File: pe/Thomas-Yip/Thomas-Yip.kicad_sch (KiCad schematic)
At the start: 17 parts, among them U1 TPS563201DDCR

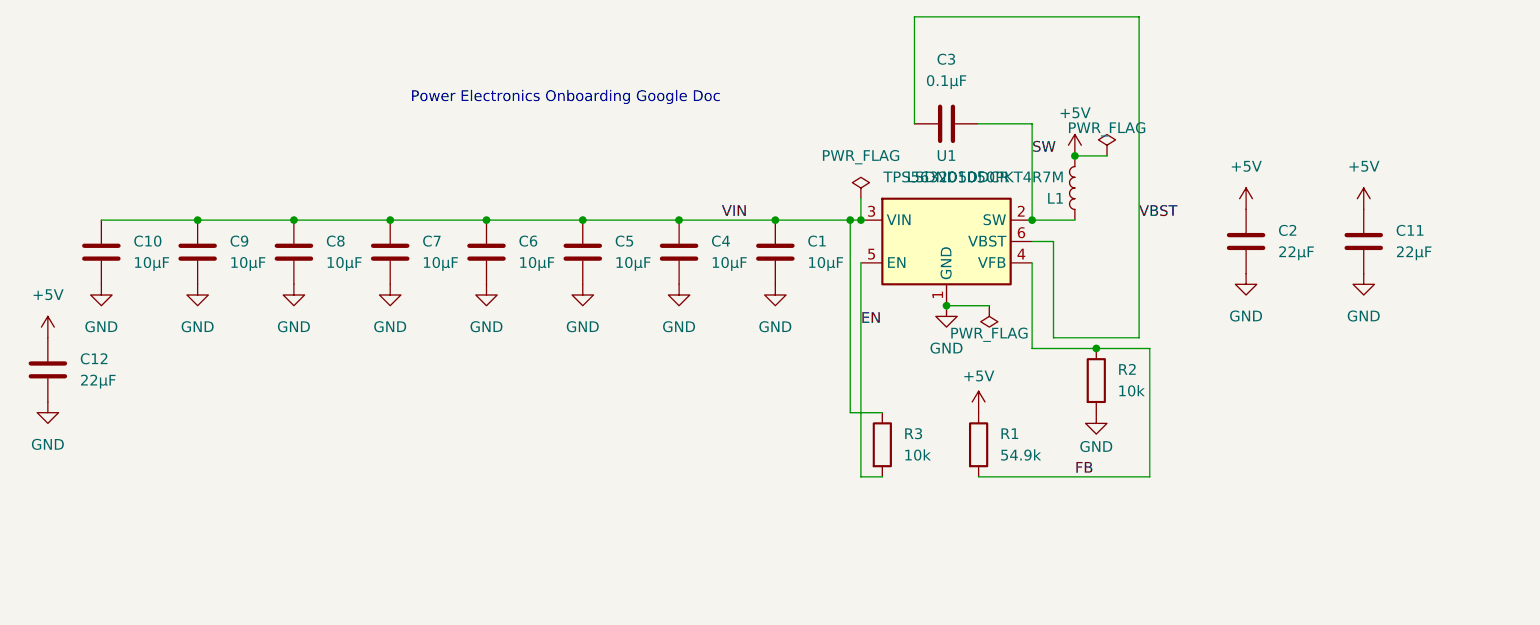
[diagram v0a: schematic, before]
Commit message: Update Thomas-Yip.kicad_sch
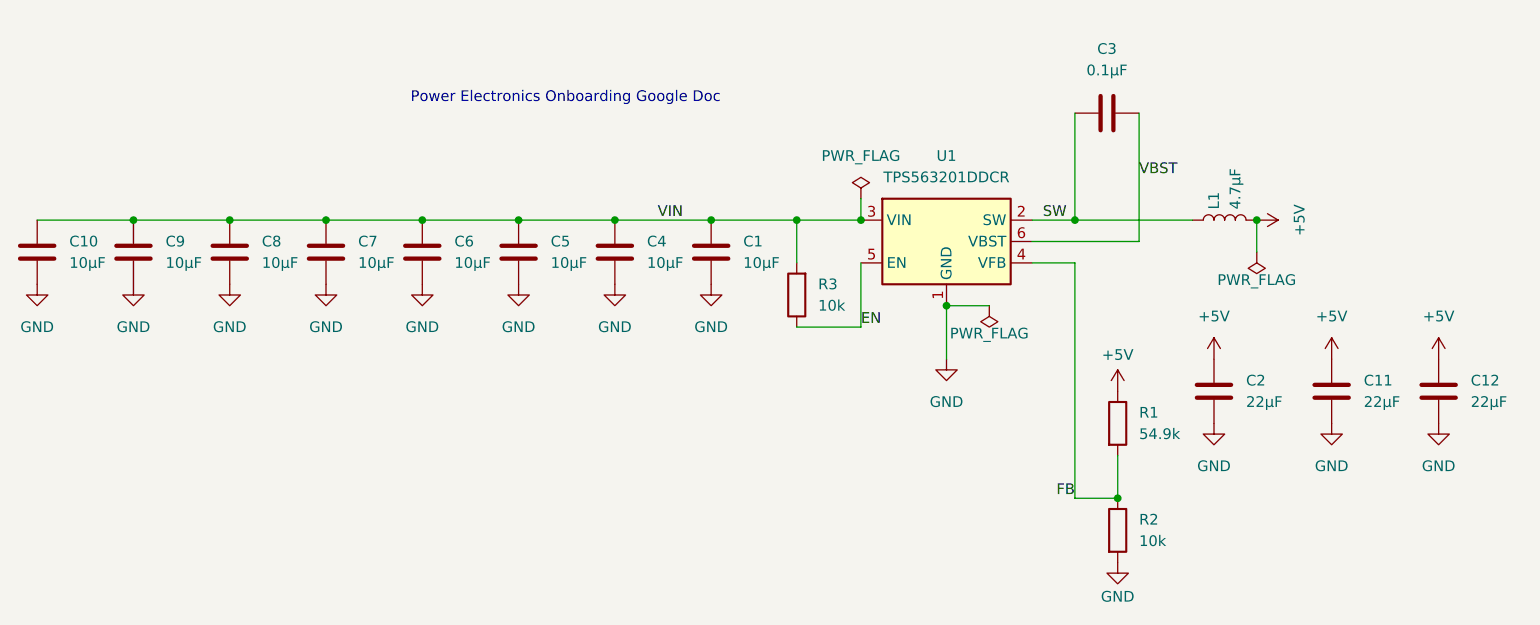
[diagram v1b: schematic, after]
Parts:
- L1: value LSDND5050PKT4R7M -> 4.7µF
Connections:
- net EN: now also R3.1; no longer R3.2
- net SW: now also C3.1; no longer C3.2
- net VBST: now also C3.2; no longer C3.1
- net VIN: now also R3.2; no longer R3.1
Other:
- moved on the sheet: C1, C10, C11, C12, C2, C3, C4, C5, C6, C7, C8, C9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
